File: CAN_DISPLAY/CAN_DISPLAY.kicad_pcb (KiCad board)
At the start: 4 copper layers, 188 x 103 mm, 130 parts, among them J1 DISPLAY, J10 DCDC 5V 3A, J11 Micro_SD_Card, J13 Prodrammer, J14 Display, J15 LED Display, J16 BME280 Module, J18 J-Link, J19 TSL2561, J2 I2C Sensor 1, J20 NMEA0183, J3 I2C Sensor 2, J4 NMEA2000, J5 Power, J6 12V, J8 DCDC 5V, J9 DCDC 5V, Q1 BC547, SW1 BOOT, SW2 RESET, U1 ESP32-DevKit, U2 ESP32-WROOM-E, U3 ISO1050DUB, U4 AMS1117-5.0, U5 ISO3080DW, U6 BME280, U7 AMS1117-3.3

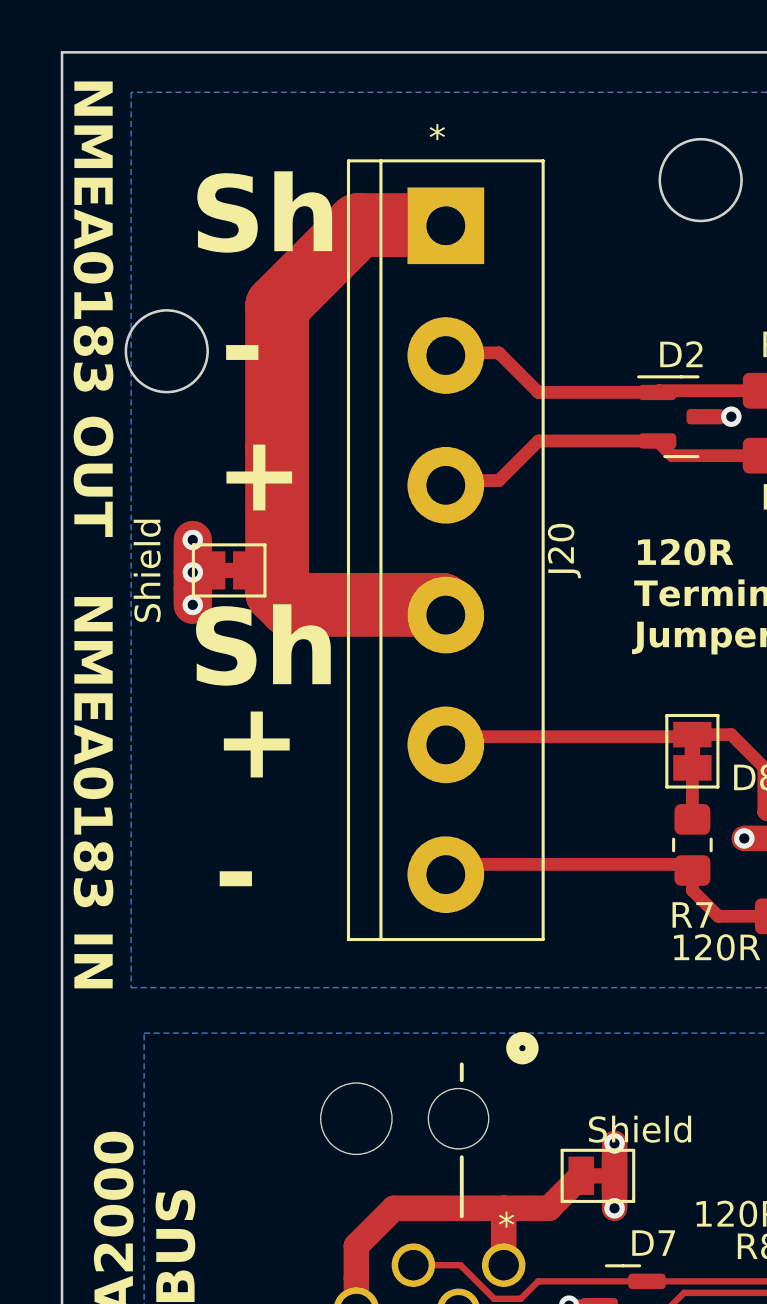
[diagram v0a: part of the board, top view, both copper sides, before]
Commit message: 1234
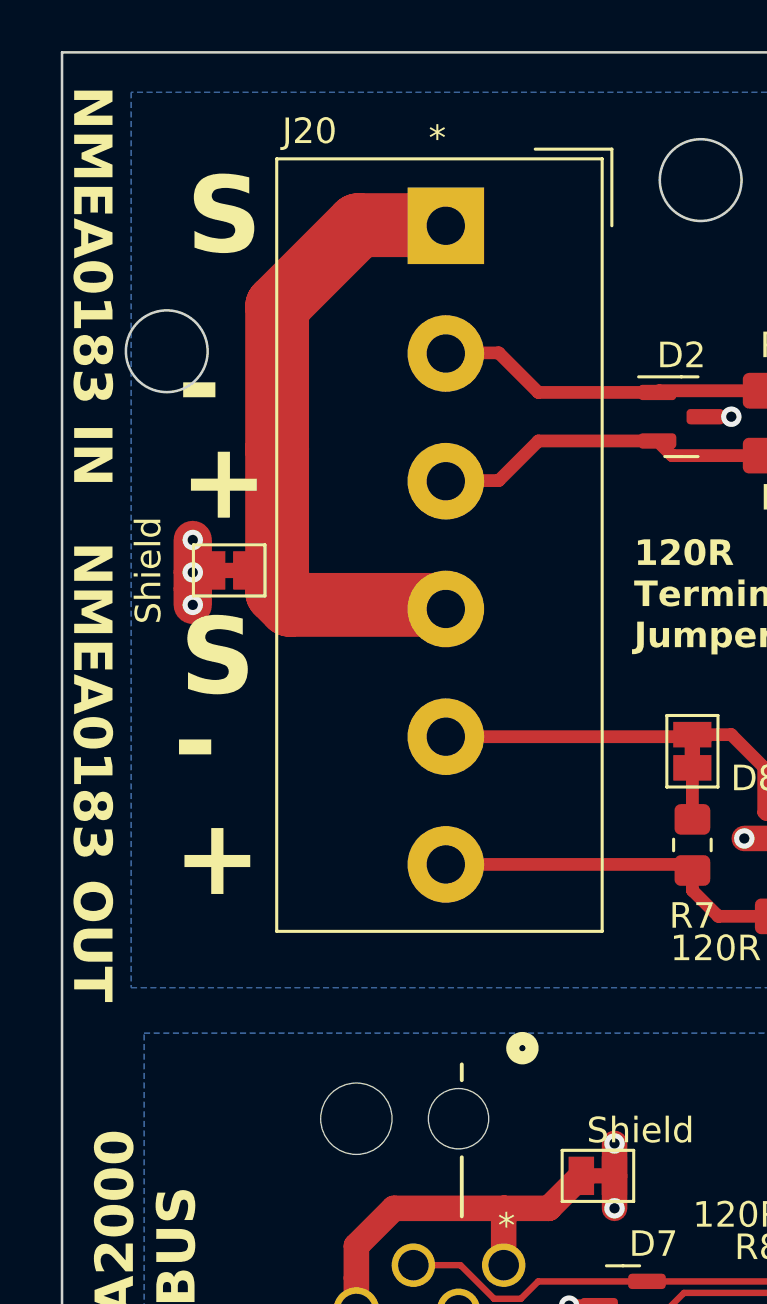
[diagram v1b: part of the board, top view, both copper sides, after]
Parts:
- J20: footprint TerminalBlock:TerminalBlock_bornier-6_P5.08mm -> TerminalBlock_Altech:Altech_AK300_1x06_P5.00mm_45-Degree
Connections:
- net /Isolated/rNMEA IN+ renamed Net-(U5-B)
- net /Isolated/rNMEA IN- renamed Net-(U5-A)
- net /Isolated/rNMEA OUT+ renamed Net-(U5-Z)
- net /Isolated/rNMEA OUT- renamed Net-(U5-Y)
- D2 pad 1: /Isolated/NMEA OUT- -> /Isolated/NMEA IN-
- D2 pad 2: /Isolated/NMEA OUT+ -> /Isolated/NMEA IN+
- D8 pad 1: /Isolated/NMEA IN- -> /Isolated/NMEA OUT+
- D8 pad 2: /Isolated/NMEA IN+ -> /Isolated/NMEA OUT-
- J20 pad 2: /Isolated/NMEA OUT- -> /Isolated/NMEA IN-
- J20 pad 3: /Isolated/NMEA OUT+ -> /Isolated/NMEA IN+
- J20 pad 5: /Isolated/NMEA IN+ -> /Isolated/NMEA OUT-
- J20 pad 6: /Isolated/NMEA IN- -> /Isolated/NMEA OUT+
- JP18 pad 2: /Isolated/NMEA IN+ -> /Isolated/NMEA OUT-
- R1 pad 2: /Isolated/NMEA IN+ -> /Isolated/NMEA OUT-
- R2 pad 2: /Isolated/NMEA IN- -> /Isolated/NMEA OUT+
- R3 pad 2: /Isolated/NMEA OUT+ -> /Isolated/NMEA IN+
- R4 pad 2: /Isolated/NMEA OUT- -> /Isolated/NMEA IN-
- R5 pad 2: /Isolated/NMEA IN+ -> /Isolated/NMEA OUT-
- R6 pad 1: /Isolated/NMEA IN- -> /Isolated/NMEA OUT+
- R7 pad 2: /Isolated/NMEA IN- -> /Isolated/NMEA OUT+
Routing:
- net /Isolated/NMEA OUT-: track 13.0 -> 33.8 mm
- net /Isolated/NMEA IN+: track 33.8 -> 13.1 mm
- net /Isolated/NMEA IN-: track 32.3 -> 13.0 mm
- net /Isolated/NMEA OUT+: track 13.1 -> 32.3 mm
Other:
- board text added: "NMEA0183 IN NMEA0183 OUT"
- board text added: "S"
- board text removed: "NMEA0183 OUT NMEA0183 IN"
- board text removed: "Sh"
